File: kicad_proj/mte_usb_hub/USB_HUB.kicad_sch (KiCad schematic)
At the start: 50 parts

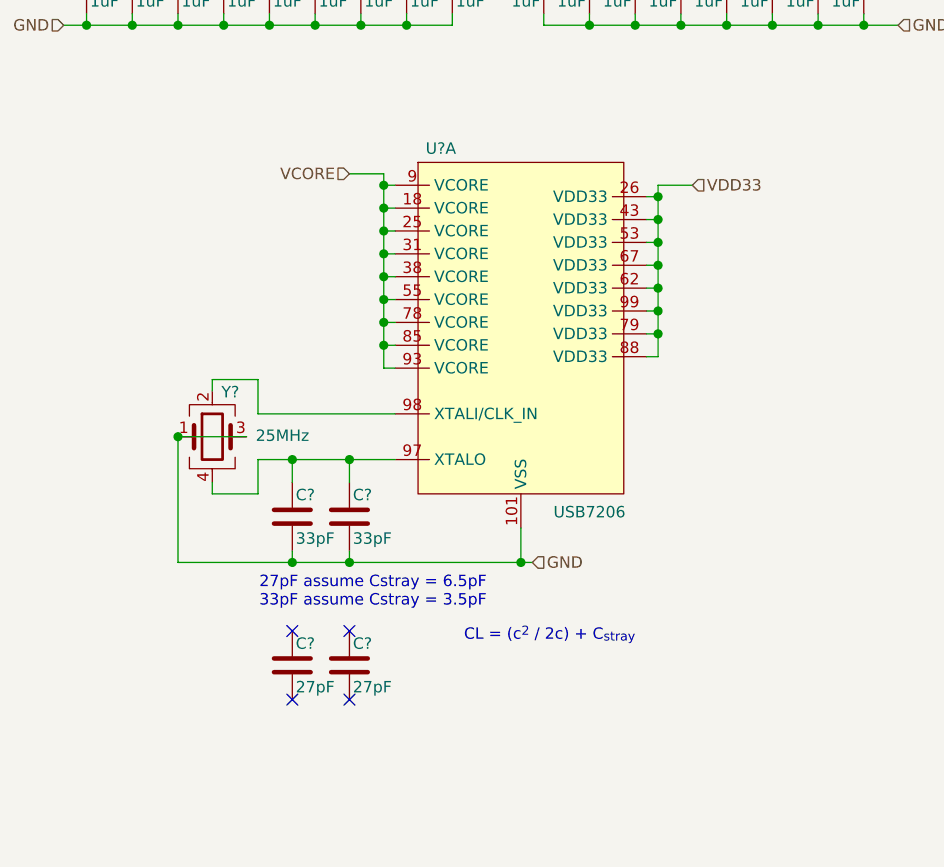
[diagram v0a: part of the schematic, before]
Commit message: Final tweaks for the video
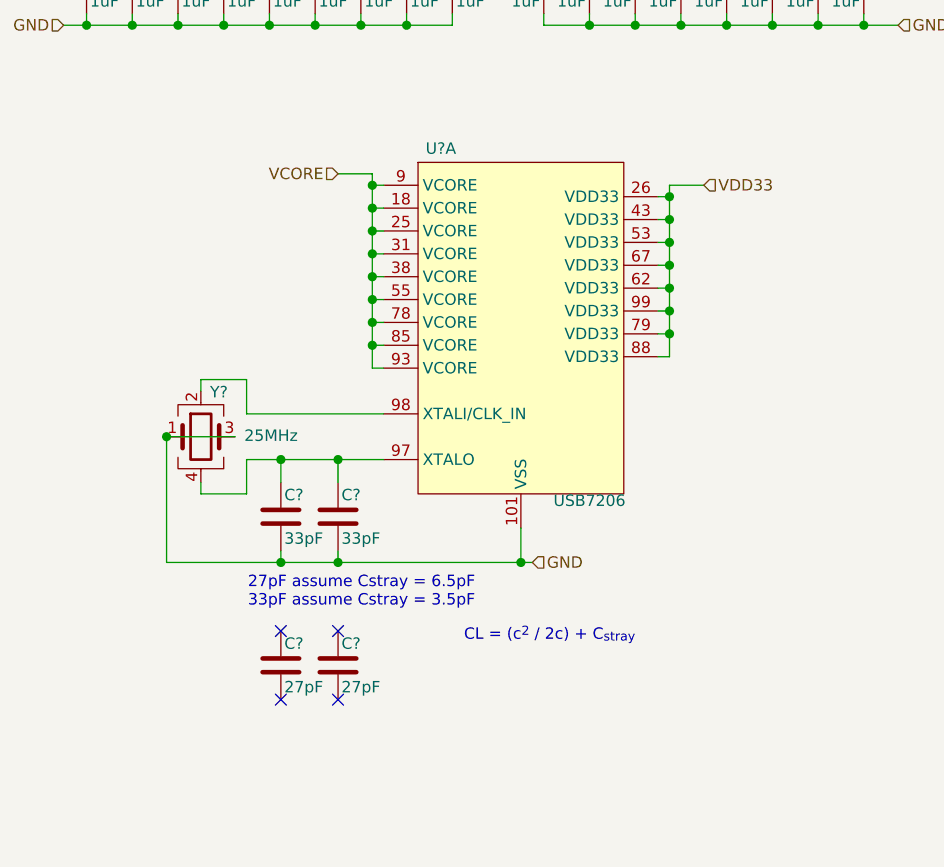
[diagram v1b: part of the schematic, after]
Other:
- moved on the sheet: C?, Y?
